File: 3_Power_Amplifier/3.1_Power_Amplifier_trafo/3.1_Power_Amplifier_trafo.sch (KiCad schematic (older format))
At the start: 11 parts, among them P1 IN_SWITCHEO, P2 OUT_CON_CAP, P3 OUT_SIN_CAP, P4 IN_FUENTE_CONM, T1 TRANSFO-SO12

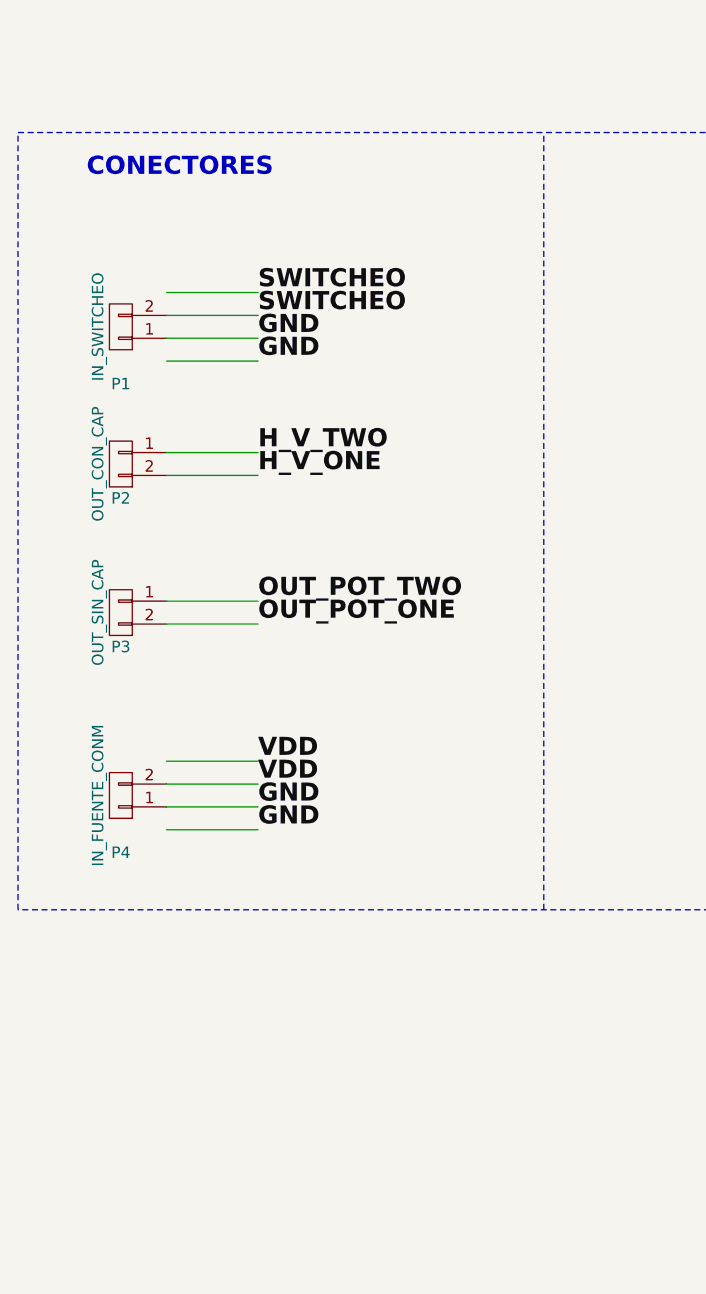
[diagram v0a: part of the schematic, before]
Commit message: AMPLIFICADOR DE POTENCIA_2 PCB_UNO
CON ISLETAS Y DISIPADORES VERTICALES
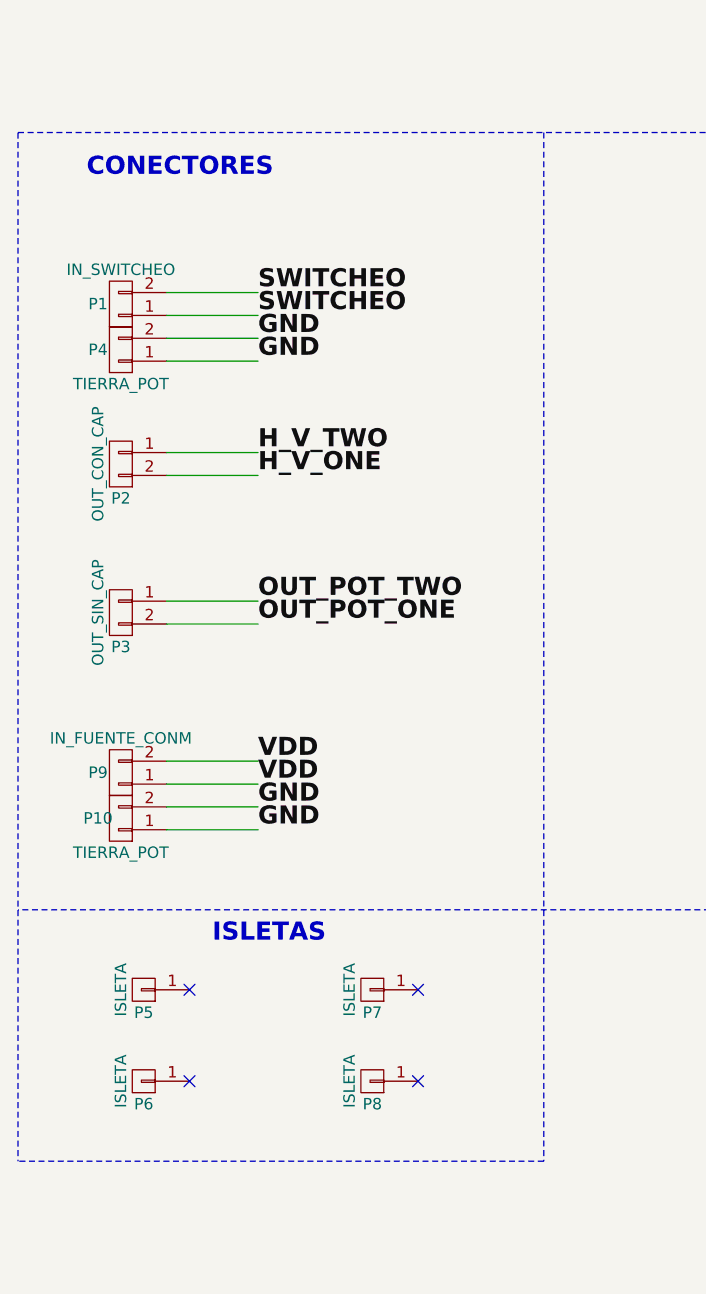
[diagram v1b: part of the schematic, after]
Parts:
- removed P4: IN_FUENTE_CONM, Sockets_MOLEX_KK-System:Socket_MOLEX-KK-RM3-96mm_Lock_4pin_straight, symbol IN_FUENTE_CONM
- added P10, P4: TIERRA_POT, Sockets_MOLEX_KK-System:Socket_MOLEX-KK-RM3-96mm_Lock_2pin_straight, symbol TIERRA_POT
- added P5, P6, P7, P8: ISLETA, libreria_Power_Amplifier_huellas:Pad_Via_5.1mm_TOR, symbol ISLETA
- added P9: IN_FUENTE_CONM, Sockets_MOLEX_KK-System:Socket_MOLEX-KK-RM3-96mm_Lock_2pin_straight, symbol IN_FUENTE_CONM
- P1: footprint Sockets_MOLEX_KK-System:Socket_MOLEX-KK-RM3-96mm_Lock_4pin_straight -> Sockets_MOLEX_KK-System:Socket_MOLEX-KK-RM3-96mm_Lock_2pin_straight
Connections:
- no-connect marks 0 -> 4
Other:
- note added: "ISLETAS"
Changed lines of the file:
@@
 	1    0    0    -1
 $EndComp
-$Comp
-L IN_FUENTE_CONM P4
-U 1 1 59CFA514
-P 1200 4000
-F 0 "P4" H 1200 4250 50  0000 C CNN
-F 1 "IN_FUENTE_CONM" V 1300 4000 50  0000 C CNN
-F 2 "Sockets_MOLEX_KK-System:Socket_MOLEX-KK-RM3-96mm_Lock_4pin_straight" H 1100 4150 50  0001 C CNN
-F 3 "" H 1200 4000 50  0000 C CNN
-	1    1200 4000
-	-1   0    0    1
-$EndComp
 Wire Notes Line
 	750  1100 11000 1100
@@
 	11000 4500 750  4500
 Wire Notes Line
-	750  4500 750  1100
+	750  1100 750  5600
 Text Notes 1050 1300 0    79   ~ 16
 CONECTORES
-$Comp
-L IN_SWITCHEO P1
-U 1 1 59CFAC64
-P 1200 1950
-F 0 "P1" H 1200 2200 50  0000 C CNN
-F 1 "IN_SWITCHEO" V 1300 1950 50  0000 C CNN
-F 2 "Sockets_MOLEX_KK-System:Socket_MOLEX-KK-RM3-96mm_Lock_4pin_straight" H 1100 2100 50  0001 C CNN
-F 3 "" H 1200 1950 50  0000 C CNN
-	1    1200 1950
-	-1   0    0    1
-$EndComp
 Text Notes 4100 1550 0    79   ~ 16
 ARREGLO DE CAPACITORES \nTANQUE LC
@@
 	6900 1100 6900 6100
 Wire Notes Line
-	3050 4500 3050 1100
+	3050 1100 3050 5600
 Text Label 7800 3150 0    79   ~ 16
 VDD
@@
 	-1   0    0    1
 $EndComp
+$Comp
+L ISLETA P5
+U 1 1 59D07AFC
+P 1300 4850
+F 0 "P5" H 1300 4950 50  0000 C CNN
+F 1 "ISLETA" V 1400 4850 50  0000 C CNN
+F 2 "libreria_Power_Amplifier_huellas:Pad_Via_5.1mm_TOR" H 1200 4850 50  0001 C CNN
+F 3 "" H 1300 4950 50  0000 C CNN
+	1    1300 4850
+	-1   0    0    1
+$EndComp
+$Comp
+L ISLETA P6
+U 1 1 59D07C9B
+P 1300 5250
+F 0 "P6" H 1300 5350 50  0000 C CNN
+F 1 "ISLETA" V 1400 5250 50  0000 C CNN
+F 2 "libreria_Power_Amplifier_huellas:Pad_Via_5.1mm_TOR" H 1200 5250 50  0001 C CNN
+F 3 "" H 1300 5350 50  0000 C CNN
+	1    1300 5250
+	-1   0    0    1
+$EndComp
+$Comp
+L ISLETA P7
+U 1 1 59D07CDC
+P 2300 4850
+F 0 "P7" H 2300 4950 50  0000 C CNN
+F 1 "ISLETA" V 2400 4850 50  0000 C CNN
+F 2 "libreria_Power_Amplifier_huellas:Pad_Via_5.1mm_TOR" H 2200 4850 50  0001 C CNN
+F 3 "" H 2300 4950 50  0000 C CNN
+	1    2300 4850
+	-1   0    0    1
+$EndComp
+$Comp
+L ISLETA P8
+U 1 1 59D07D6C
+P 2300 5250
+F 0 "P8" H 2300 5350 50  0000 C CNN
+F 1 "ISLETA" V 2400 5250 50  0000 C CNN
+F 2 "libreria_Power_Amplifier_huellas:Pad_Via_5.1mm_TOR" H 2200 5250 50  0001 C CNN
+F 3 "" H 2300 5350 50  0000 C CNN
+	1    2300 5250
+	-1   0    0    1
+$EndComp
+NoConn ~ 2500 4850
+NoConn ~ 2500 5250
+NoConn ~ 1500 5250
+NoConn ~ 1500 4850
+Wire Notes Line
+	3050 5600 750  5600
+Text Notes 1600 4650 0    79   ~ 16
+ISLETAS
+$Comp
+L IN_SWITCHEO P1
+U 1 1 59D04926
+P 1200 1850
+F 0 "P1" H 1300 1850 50  0000 C CNN
+F 1 "IN_SWITCHEO" H 1200 1700 50  0000 C CNN
+F 2 "Sockets_MOLEX_KK-System:Socket_MOLEX-KK-RM3-96mm_Lock_2pin_straight" H 1100 1900 50  0001 C CNN
+F 3 "" H 1200 1850 50  0000 C CNN
+	1    1200 1850
+	-1   0    0    1
+$EndComp
+$Comp
+L TIERRA_POT P4
+U 1 1 59D04A46
+P 1200 2050
+F 0 "P4" H 1300 2050 50  0000 C CNN
+F 1 "TIERRA_POT" H 1200 2200 50  0000 C CNN
+F 2 "Sockets_MOLEX_KK-System:Socket_MOLEX-KK-RM3-96mm_Lock_2pin_straight" H 1100 2100 50  0001 C CNN
+F 3 "" H 1200 2050 50  0000 C CNN
+	1    1200 2050
+	-1   0    0    1
+$EndComp
+$Comp
+L IN_FUENTE_CONM P9
+U 1 1 59D05006
+P 1200 3900
+F 0 "P9" H 1300 3900 50  0000 C CNN
+F 1 "IN_FUENTE_CONM" H 1200 3750 50  0000 C CNN
+F 2 "Sockets_MOLEX_KK-System:Socket_MOLEX-KK-RM3-96mm_Lock_2pin_straight" H 1100 3950 50  0001 C CNN
+F 3 "" H 1200 3900 50  0000 C CNN
+	1    1200 3900
+	-1   0    0    1
+$EndComp
+$Comp
+L TIERRA_POT P10
+U 1 1 59D050DC
+P 1200 4100
+F 0 "P10" H 1300 4100 50  0000 C CNN
+F 1 "TIERRA_POT" H 1200 4250 50  0000 C CNN
+F 2 "Sockets_MOLEX_KK-System:Socket_MOLEX-KK-RM3-96mm_Lock_2pin_straight" H 1100 4150 50  0001 C CNN
+F 3 "" H 1200 4100 50  0000 C CNN
+	1    1200 4100
+	-1   0    0    1
+$EndComp
